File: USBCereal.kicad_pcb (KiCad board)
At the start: 2 copper layers, 25.1 x 19.6 mm, 18 parts, among them J1 USB_C, J2 Conn_01x06, U1 XC6206P332MR, U2 CH340C

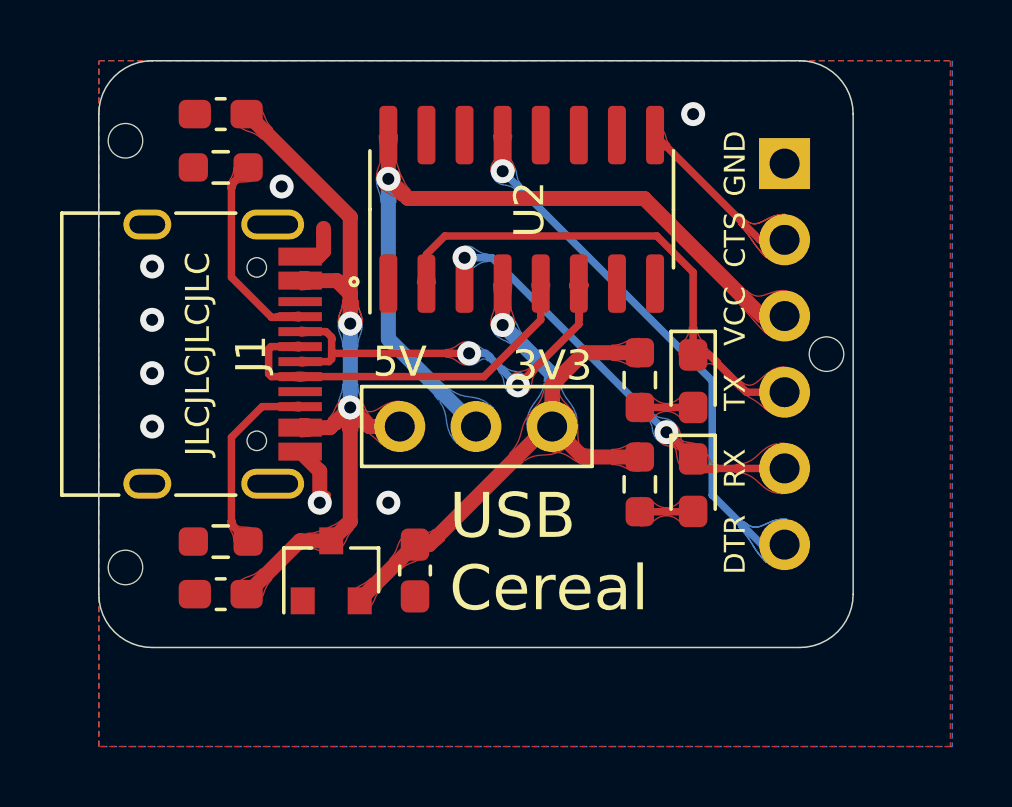
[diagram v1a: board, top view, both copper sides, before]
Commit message: update to kicad 6.0
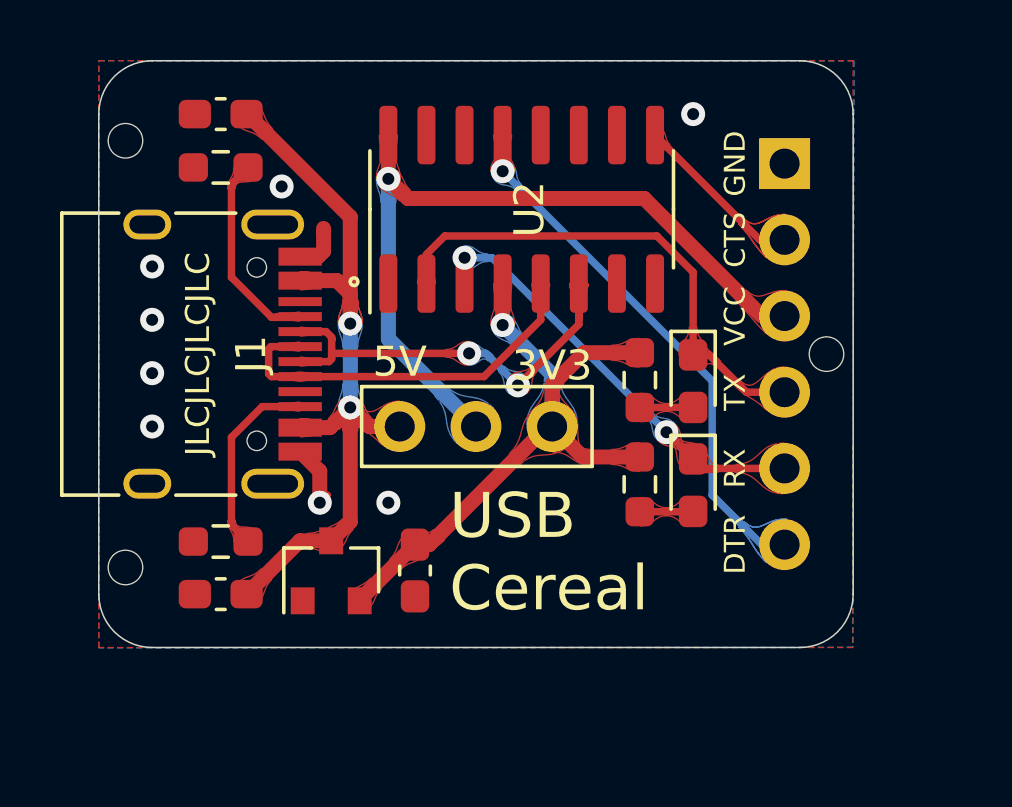
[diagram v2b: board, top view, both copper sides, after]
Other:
- net class Default removed
- net class VCC removed
